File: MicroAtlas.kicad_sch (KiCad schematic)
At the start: 37 parts, among them J1 TAGCONNECT, J2 Conn_01x02, J3 Conn_01x04_MountingPin, J4 SMA_Edgelaunch, J5 UFL, U1 NEO-F9P, U2 RAK3172-xx-43-SM-xI, U3 TPS7A2033PDBVR, U4 W25Q32JVZP, U5 TPS2116DRL, U6 LSM6DSV320XTR

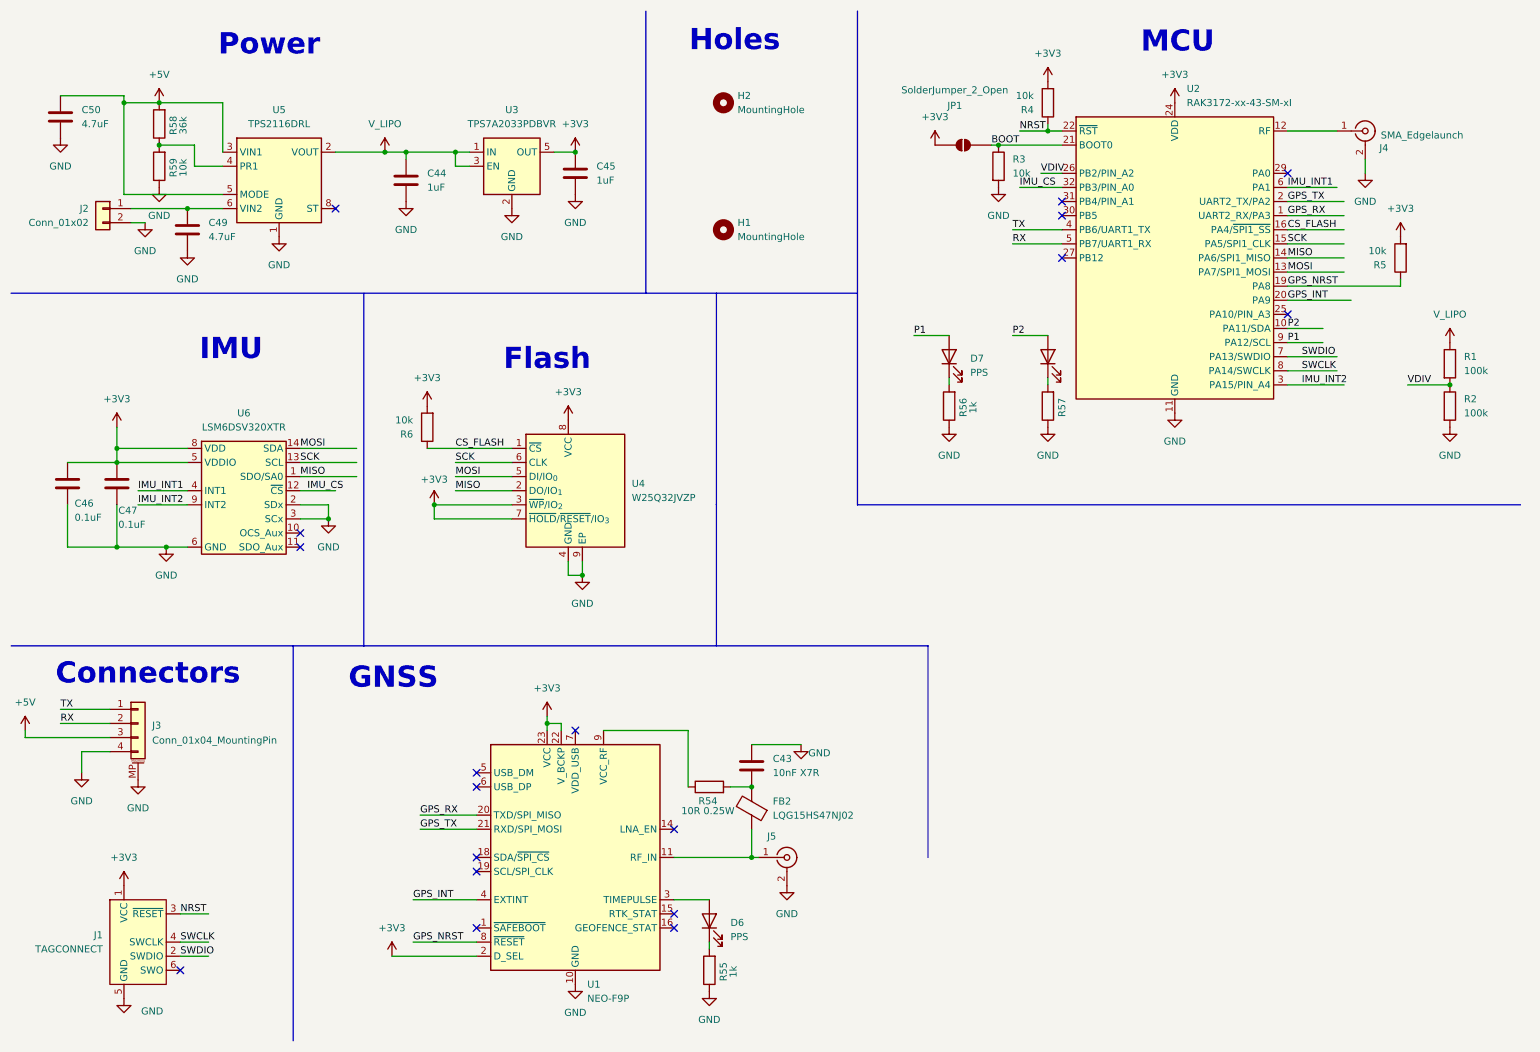
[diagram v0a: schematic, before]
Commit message: prod v2.0
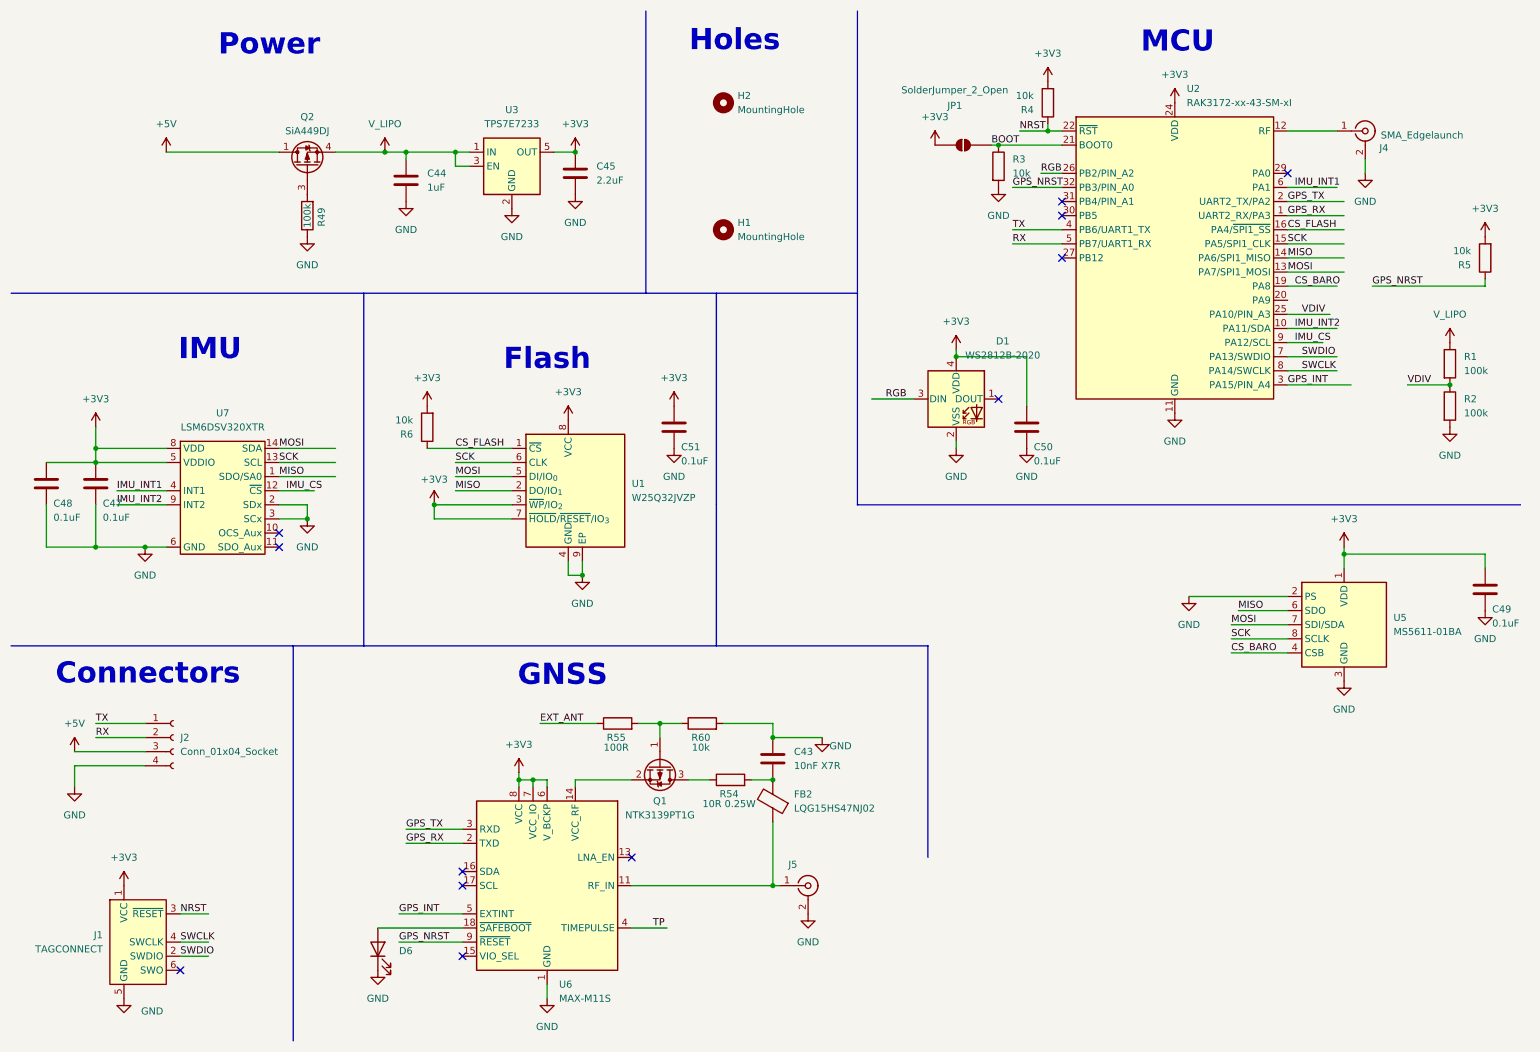
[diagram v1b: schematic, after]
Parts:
- removed C46: 0.1uF, Capacitor_SMD:C_0402_1005Metric, symbol Device:C
- removed D7, D8: PPS, LED_SMD:LED_0402_1005Metric, symbol Device:LED
- removed J2: Conn_01x02, Connector_JST:JST_PH_S2B-PH-K_1x02_P2.00mm_Horizontal, symbol Connector_Generic:Conn_01x02
- removed J3: Conn_01x04_MountingPin, Connector_JST:JST_SH_SM04B-SRSS-TB_1x04-1MP_P1.00mm_Horizontal, symbol Connector_Generic_MountingPin:Conn_01x04_MountingPin
- removed R56, R57: 1k, Resistor_SMD:R_0402_1005Metric, symbol Device:R
- removed R58: 36k, Resistor_SMD:R_0402_1005Metric, symbol Device:R
- removed R59: 10k, Resistor_SMD:R_0402_1005Metric, symbol Device:R
- removed U1: NEO-F9P, RF_GPS:ublox_NEO, symbol RF_GPS:NEO-M8P
- removed U4: W25Q32JVZP, Package_SON:WSON-8-1EP_6x5mm_P1.27mm_EP3.4x4.3mm, symbol Memory_Flash:W25Q32JVZP
- removed U5: TPS2116DRL, Package_TO_SOT_SMD:SOT-583-8, symbol Power_Management:TPS2116DRL
- removed U6: LSM6DSV320XTR, PCM_SparkFun-Sensor:ST_LGA-14L_2.5x3.0mm_P0.5mm_4x3, symbol PCM_SparkFun-Sensor:LSM6DSOX
- added C48, C51: 0.1uF, Capacitor_SMD:C_0402_1005Metric, symbol Device:C
- added D1: WS2812B-2020, LED_SMD:LED_WS2812B-2020_PLCC4_2.0x2.0mm, symbol LED:WS2812B-2020
- added J2: Conn_01x04_Socket, FCU2025Lib:CONN_2200980000-SD_04P_MOL, symbol Connector:Conn_01x04_Socket
- added Q1: NTK3139PT1G, Package_TO_SOT_SMD:SOT-723, symbol Transistor_FET:AO3401A
- added Q2: SiA449DJ, Package_TO_SOT_SMD:Vishay_PowerPAK_SC70-6L_Single, symbol Transistor_FET:SiA449DJ
- added R49: 100k, Resistor_SMD:R_0402_1005Metric, symbol Device:R
- added R60: 10k, Resistor_SMD:R_0402_1005Metric, symbol Device:R
- added U1: W25Q32JVZP, Package_SON:WSON-8-1EP_6x5mm_P1.27mm_EP3.4x4.3mm, symbol Memory_Flash:W25Q32JVZP
- added U5: MS5611-01BA, Package_LGA:LGA-8_3x5mm_P1.25mm, symbol Sensor_Pressure:MS5611-01BA
- added U6: MAX-M11S, RF_GPS:ublox_MAX, symbol RF_GPS:MAX-M10S
- added U7: LSM6DSV320XTR, PCM_SparkFun-Sensor:ST_LGA-14L_2.5x3.0mm_P0.5mm_4x3, symbol PCM_SparkFun-Sensor:LSM6DSOX
- C45: value 1uF -> 2.2uF
- C49, C50: value 4.7uF -> 0.1uF
- R55: value 1k -> 100R
- U3: value TPS7A2033PDBVR -> TPS7E7233
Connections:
- net P1 is gone; now on net IMU_CS: U2.9 (PA12/SCL)
- net P2 is gone; now on net IMU_INT2: U2.10 (PA11/SDA)
- net +3V3: now also C49.2, C50.2, C48.2, C51.2, D1.4 (VDD), U1.3 (~{WP}/IO_{2}), U1.7 (~{HOLD}/~{RESET}/IO_{3}), U1.8 (VCC), U5.1 (VDD), U6.6 (V_BCKP), U6.7 (VCC_IO), U6.8 (VCC), U7.5 (VDDIO), U7.8 (VDD)
- net +5V: now also J2.3 (Pin_3), Q2.1 (D); no longer C50.2
- net CS_FLASH: now also U1.1 (~{CS})
- net GND: now also D6.1 (K), C48.1, C51.1, D1.2 (VSS), J2.4 (Pin_4), R49.1, R60.2, U1.4 (GND), U1.9 (EP), U5.2 (PS), U5.3 (GND), U6.1 (GND), U6.10 (GND), U6.12 (GND), U7.2 (SDx), U7.3 (SCx), U7.6 (GND), U7.7 (GND); no longer R55.1
- net GPS_INT: now also U2.3 (PA15/PIN_A4), U6.5 (EXTINT); no longer U2.20 (PA9)
- net GPS_NRST: now also U2.32 (PB3/PIN_A0), U6.9 (~{RESET}); no longer U2.19 (PA8)
- net GPS_RX: now also U6.2 (TXD)
- net GPS_TX: now also U6.3 (RXD)
- net IMU_CS: now also U7.12 (~{CS}); no longer U2.32 (PB3/PIN_A0)
- net IMU_INT1: now also U7.4 (INT1)
- net IMU_INT2: now also U7.9 (INT2); no longer U2.3 (PA15/PIN_A4)
- net MISO: now also U1.2 (DO/IO_{1}), U5.6 (SDO), U7.1 (SDO/SA0)
- net MOSI: now also U1.5 (DI/IO_{0}), U5.7 (SDI/SDA), U7.14 (SDA)
- net RX: now also J2.2 (Pin_2)
- net SCK: now also U1.6 (CLK), U5.8 (SCLK), U7.13 (SCL)
- net TX: now also J2.1 (Pin_1)
- net VDIV: now also U2.25 (PA10/PIN_A3); no longer U2.26 (PB2/PIN_A2)
- net V_LIPO: now also Q2.4 (S)
- net at R54.1: now also Q1.3 (D)
- net at FB2.1, J5.1 (In): now also U6.11 (RF_IN)
- net at D6.2 (A): now also U6.18 (~{SAFEBOOT})
- net at R55.2: now also Q1.1 (G), R60.1; no longer D6.1 (K)
- new net: Q1.2 (S), U6.14 (VCC_RF)
- new net: Q2.3 (G), R49.2
- new net CS_BARO: U2.19 (PA8), U5.4 (CSB), U5.5 (CSB)
- new net EXT_ANT: R55.1
- new net RGB: D1.3 (DIN), U2.26 (PB2/PIN_A2)
- new net TP: U6.4 (TIMEPULSE)
- no-connect marks 18 -> 12
